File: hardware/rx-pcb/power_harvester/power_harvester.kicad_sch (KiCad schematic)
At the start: 41 parts, among them J1 Conn_Coaxial_Small, J2 Conn_01x02_Pin, J3 Conn_Coaxial_Small, J4 Conn_Coaxial_Small

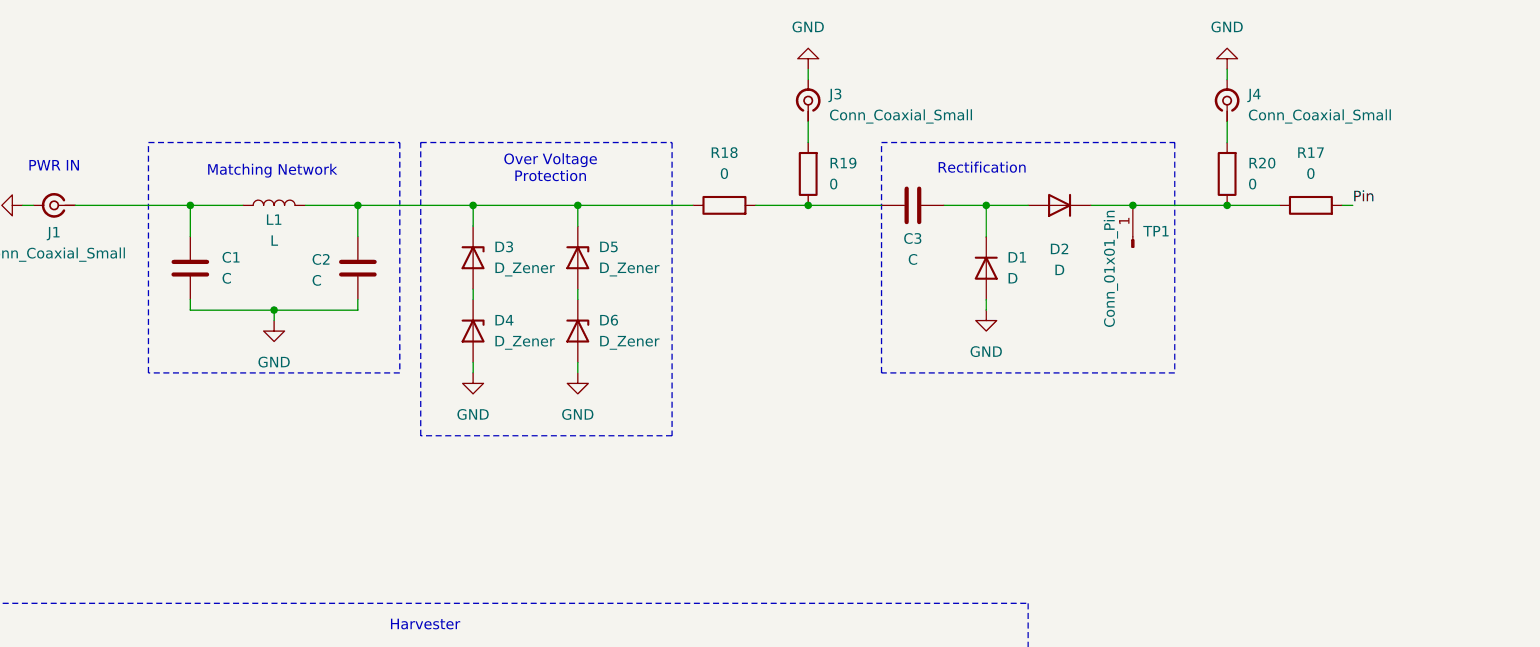
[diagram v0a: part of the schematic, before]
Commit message: power harvester updates and cleanup
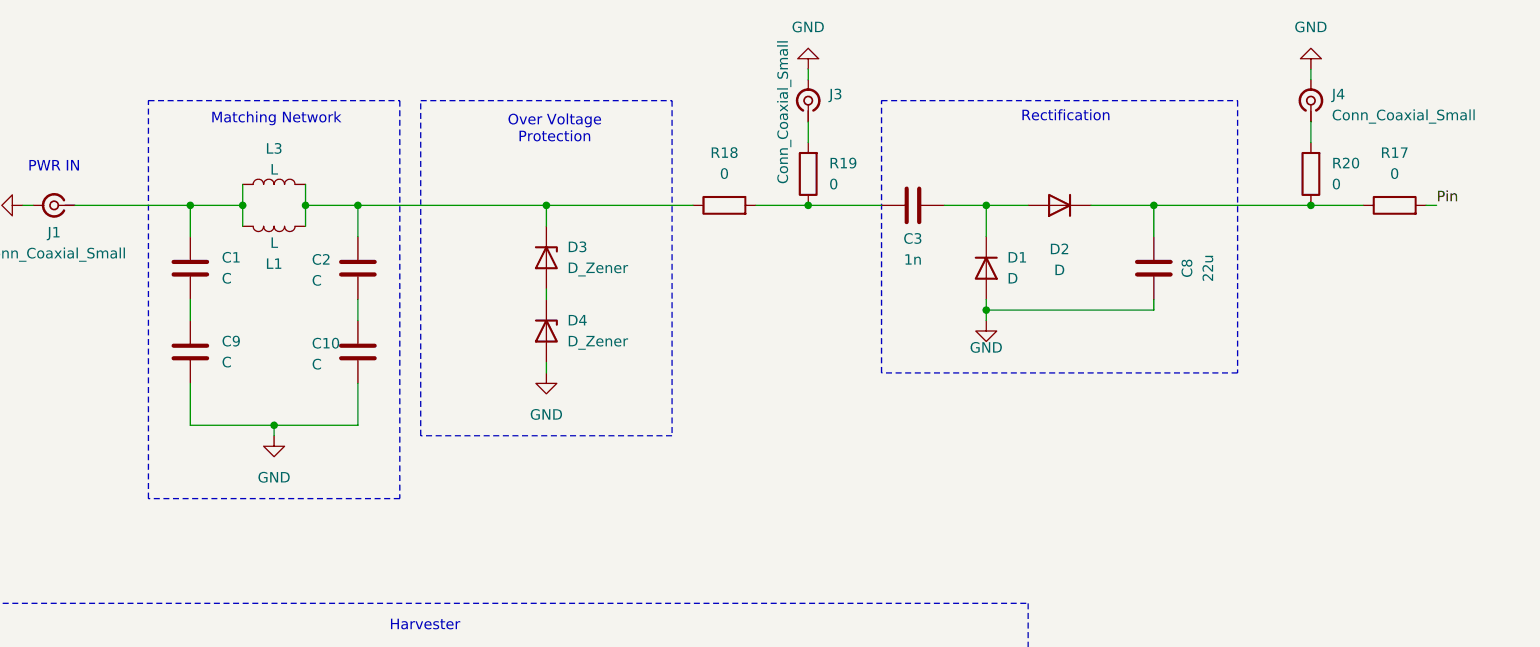
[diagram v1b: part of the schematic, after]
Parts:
- removed D5, D6: D_Zener, Capacitor_SMD:C_0201_0603Metric, symbol Device:D_Zener
- removed TP1: Conn_01x01_Pin, Connector_PinHeader_2.54mm:PinHeader_1x01_P2.54mm_Vertical, symbol Connector:Conn_01x01_Pin
- added C10, C9: C, Capacitor_SMD:C_0603_1608Metric_Pad1.08x0.95mm_HandSolder, symbol Device:C
- added C8: 22u, Capacitor_SMD:C_0603_1608Metric_Pad1.08x0.95mm_HandSolder, symbol Device:C
- added L3: L, Inductor_SMD:L_0805_2012Metric_Pad1.05x1.20mm_HandSolder, symbol Device:L
- C1, C2, C4, C5, C6: footprint Capacitor_SMD:C_0805_2012Metric_Pad1.18x1.45mm_HandSolder -> Capacitor_SMD:C_0603_1608Metric_Pad1.08x0.95mm_HandSolder
- C3: value C -> 1n; footprint Capacitor_SMD:C_0805_2012Metric_Pad1.18x1.45mm_HandSolder -> Capacitor_SMD:C_0603_1608Metric_Pad1.08x0.95mm_HandSolder
- J3, J4: footprint (none) -> Connector_PinHeader_2.54mm:PinHeader_1x02_P2.54mm_Vertical
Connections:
- net GND: now also C10.2, C8.1, C9.2; no longer C1.2, C2.2
- net at D2.1 (K), R17.1, R20.1: now also C8.2
- net at C2.1, D3.1 (K), R18.1: now also L1.1, L3.2; no longer L1.2
- net at C1.1, J1.1 (In): now also L1.2, L3.1; no longer L1.1
- new net: C10.1, C2.2
- new net: C1.2, C9.1
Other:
- moved on the sheet: D3, D4, J4, L1, R17, R20
